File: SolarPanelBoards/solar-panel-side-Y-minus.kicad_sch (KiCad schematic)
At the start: 52 parts, among them J1 Conn_01x06, Q1 MBT2222ADW1T1, Q2 MBT2222ADW1T1, Q3 BSS138DWQ-7, Q4 BSS138DWQ-7, U1 OPT3001DNPT, U2 DRV8830DGQR

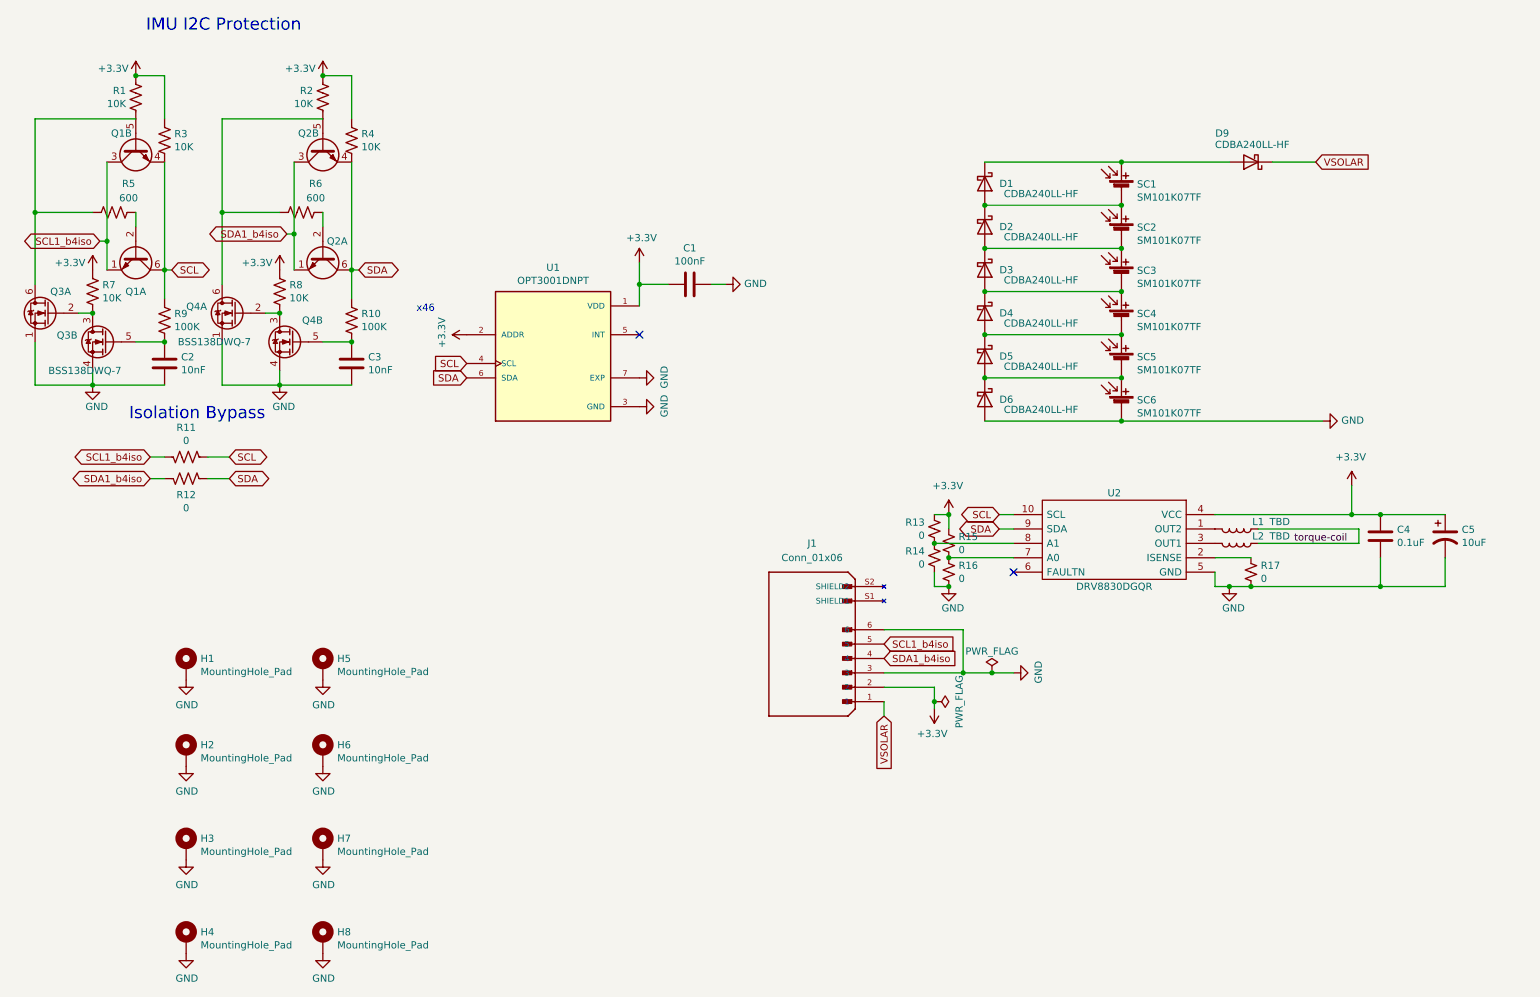
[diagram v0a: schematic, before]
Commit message: Y minus updates
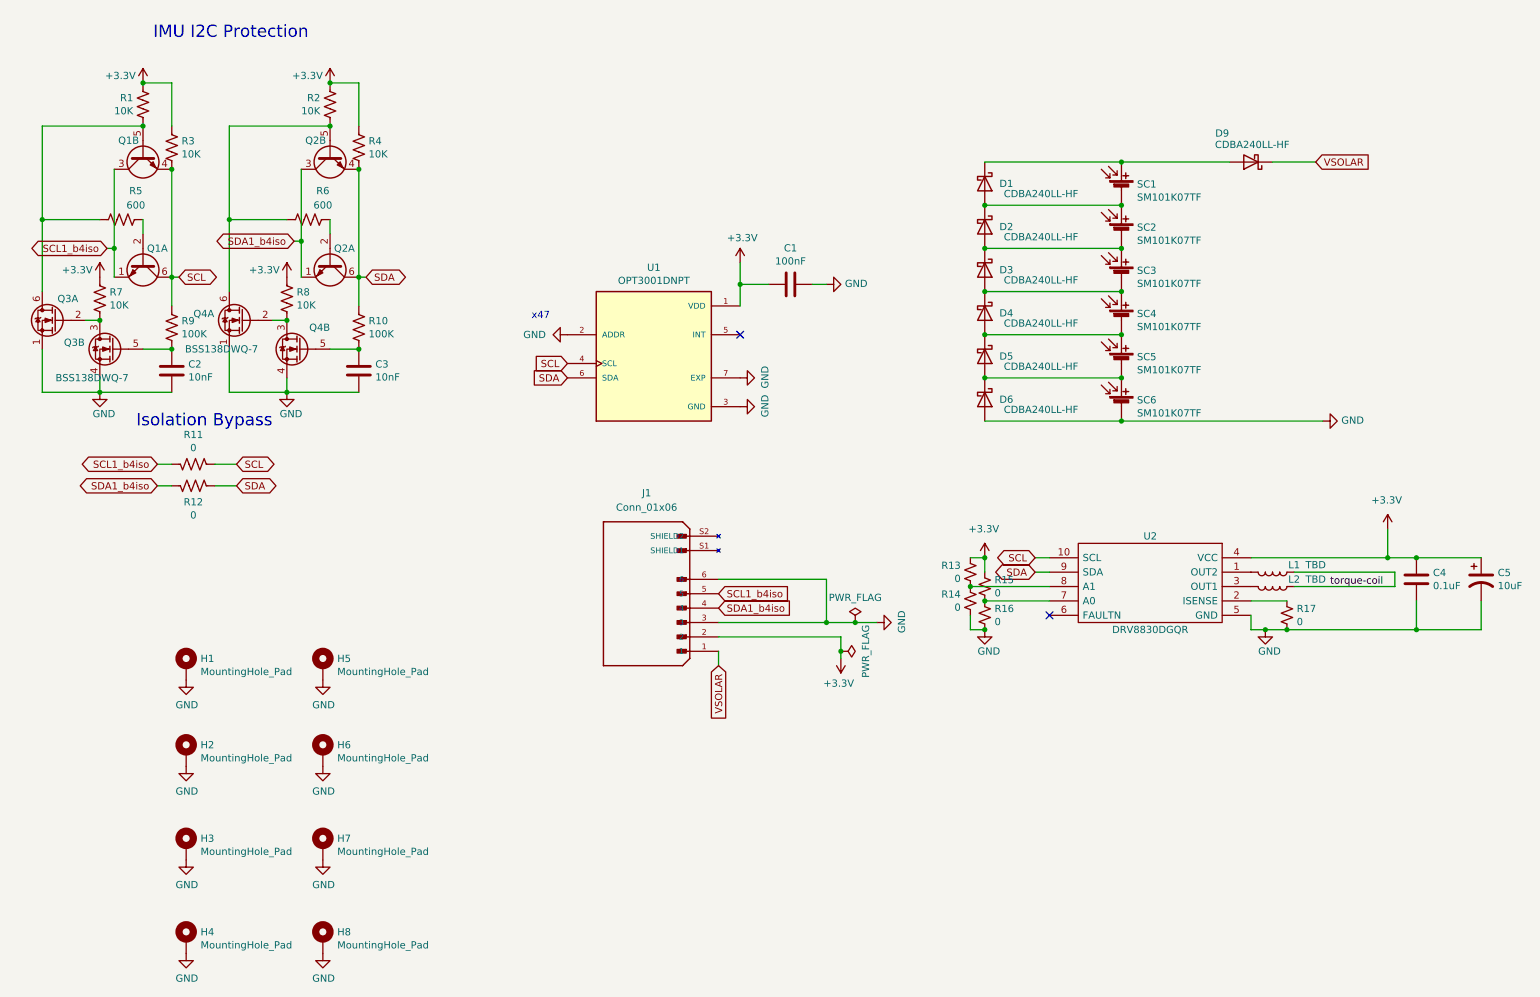
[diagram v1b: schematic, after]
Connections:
- net +3V3: no longer U1.2 (ADDR)
- net GND: now also U1.2 (ADDR)
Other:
- note added: "x47"
- note removed: "x46"
- company: SSI Satellite Team -> (none)
- title: SolarPanel+-Y -> (none)
- moved on the sheet: C1
